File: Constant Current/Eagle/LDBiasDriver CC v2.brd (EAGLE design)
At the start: 44.8 x 22.9 mm, 24 parts, among them IC1 MCP1703-5002E/DB, IC3 LM358D, U1 MCP4726A0

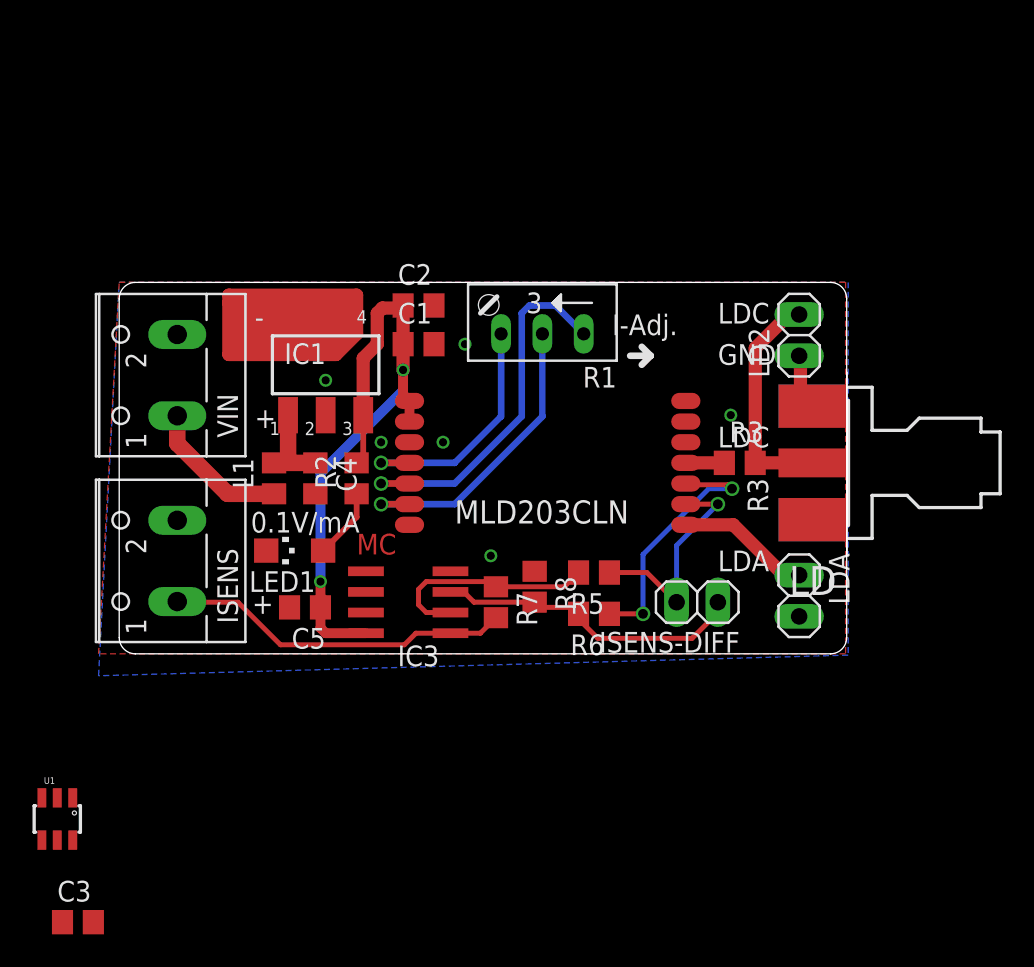
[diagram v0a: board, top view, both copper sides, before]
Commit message: updates
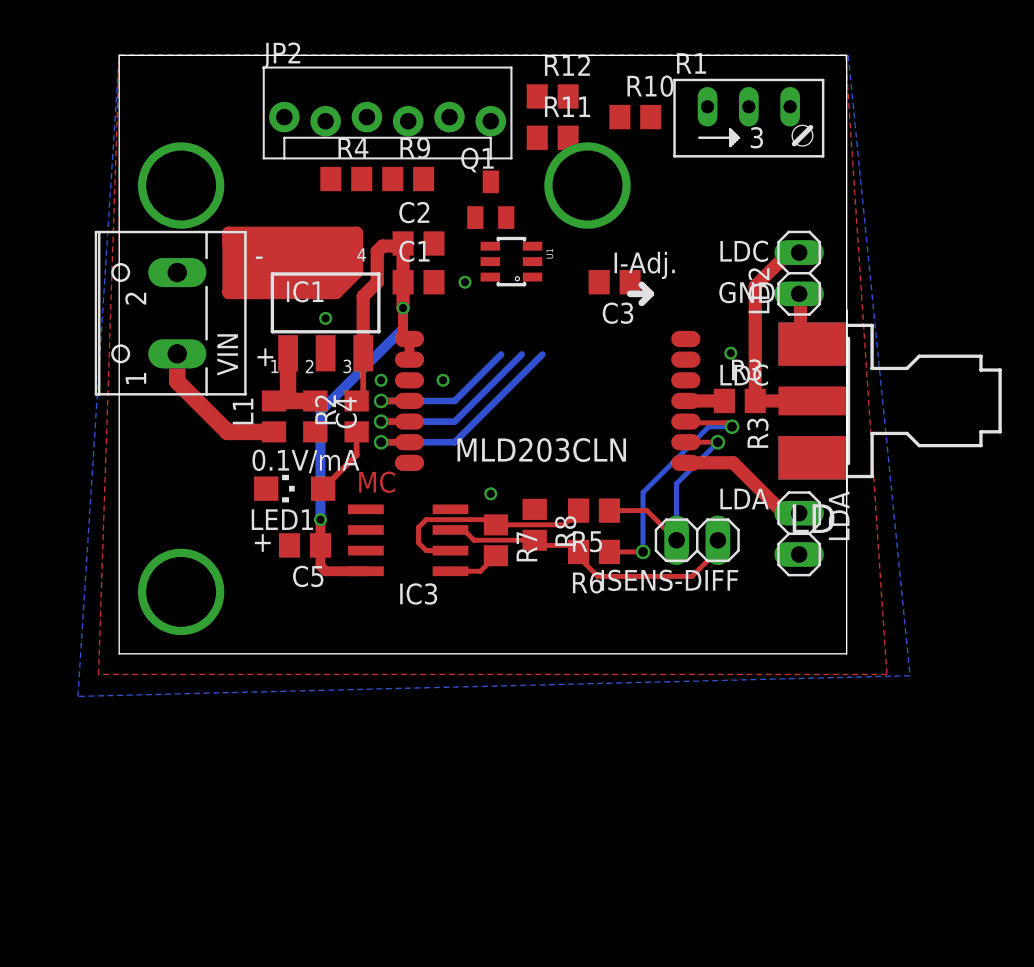
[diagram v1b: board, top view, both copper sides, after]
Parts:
- removed ISENS: (no value), con-wago-500:W237-102
- added JP2: (no value), SparkFun-Connectors:MOLEX-1X6_LOCK
- added Q1: (no value), adafruit:SOT23
- added R10, R12, R4, R9: 4.7k, rcl:R0805
- added R11: 330, rcl:R0805
- moved C3 51.4 mm to (30.5, 22.9), turned to 180 degrees
- moved U1 44.2 mm to (24.1, 24.1), turned to 270 degrees
- moved R1 18.0 mm to (38.7, 33.0), turned to 0 degrees
- moved C2 3.81 mm to (18.4, 25.2)
- moved C4 3.81 mm to (12.1, 14.6)
- moved C5 3.81 mm to (11.4, 6.67)
- moved IC3 3.81 mm to (17.8, 6.99)
- moved ISENS-DIFF 3.81 mm to (35.6, 6.99)
- moved L1 3.81 mm to (9.53, 14.6)
- moved LED1 3.81 mm to (10.8, 10.2)
- moved R2 3.81 mm to (14.6, 14.6)
- moved R7 3.81 mm to (23.2, 6.99)
- moved U$1 3.81 mm to (17.9, 19.4)
- moved LDA 3.81 mm to (41.8, 7.38)
- moved R6 3.81 mm to (29.2, 6.27)
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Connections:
- removed net N$14: L1.1, VIN.1
- removed net N$18: IC3.1, ISENS.1, R7.2
- new net ISENSE: IC3.1, JP2.6, R7.2
- new net MOD: JP2.5, R11.1
- new net N$10: Q1.1, R11.2, R12.2
- new net N$13: R10.2, U1.1
- new net SCL: JP2.4, R9.2, U1.5
- new net SDA: JP2.3, R4.2, U1.4
- new net VIN: JP2.2, L1.1, VIN.1
- net +5V: now also R4.1, R9.1
- net GND: now also JP2.1, Q1.2, R12.1; no longer ISENS.2
- net N$4: now also Q1.3, R10.1; no longer U1.1
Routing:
- net N$18: track 21.4 -> 0.00 mm, vias 0 -> 3
- net N$2: track 23.2 -> 12.1 mm
- net VIN: track 0.00 -> 8.94 mm
- net N$14: track 8.94 -> 0.00 mm
- net N$4: track 19.0 -> 13.9 mm
- net N$5: track 15.4 -> 10.3 mm
- net ISENSE: track 0.00 -> 3.19 mm
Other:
- board size 44.8 x 22.9 mm -> 44.8 x 36.8 mm
- board text added: "v2 2017"
- board text removed: "v1.1 2016"
